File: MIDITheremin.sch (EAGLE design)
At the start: 104 parts, among them IC1 TL072P, IC2 TL072P, J1 DCJ0202, T1 2N3904, T2 2N3904, T3 2N3904, T4 2N3904, T5 2N3904

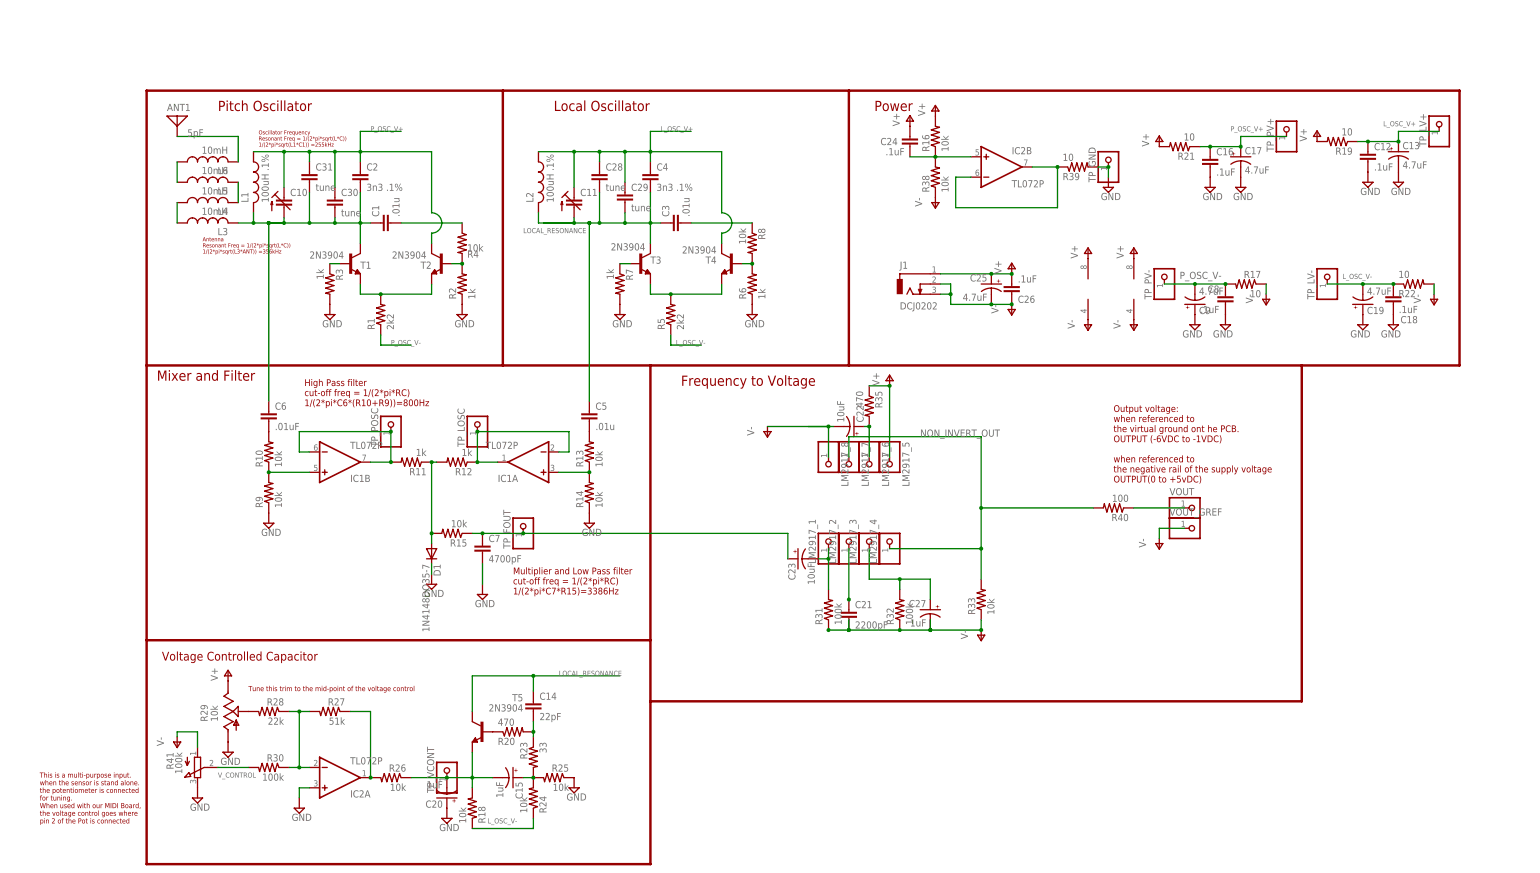
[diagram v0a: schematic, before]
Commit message: Add files via upload
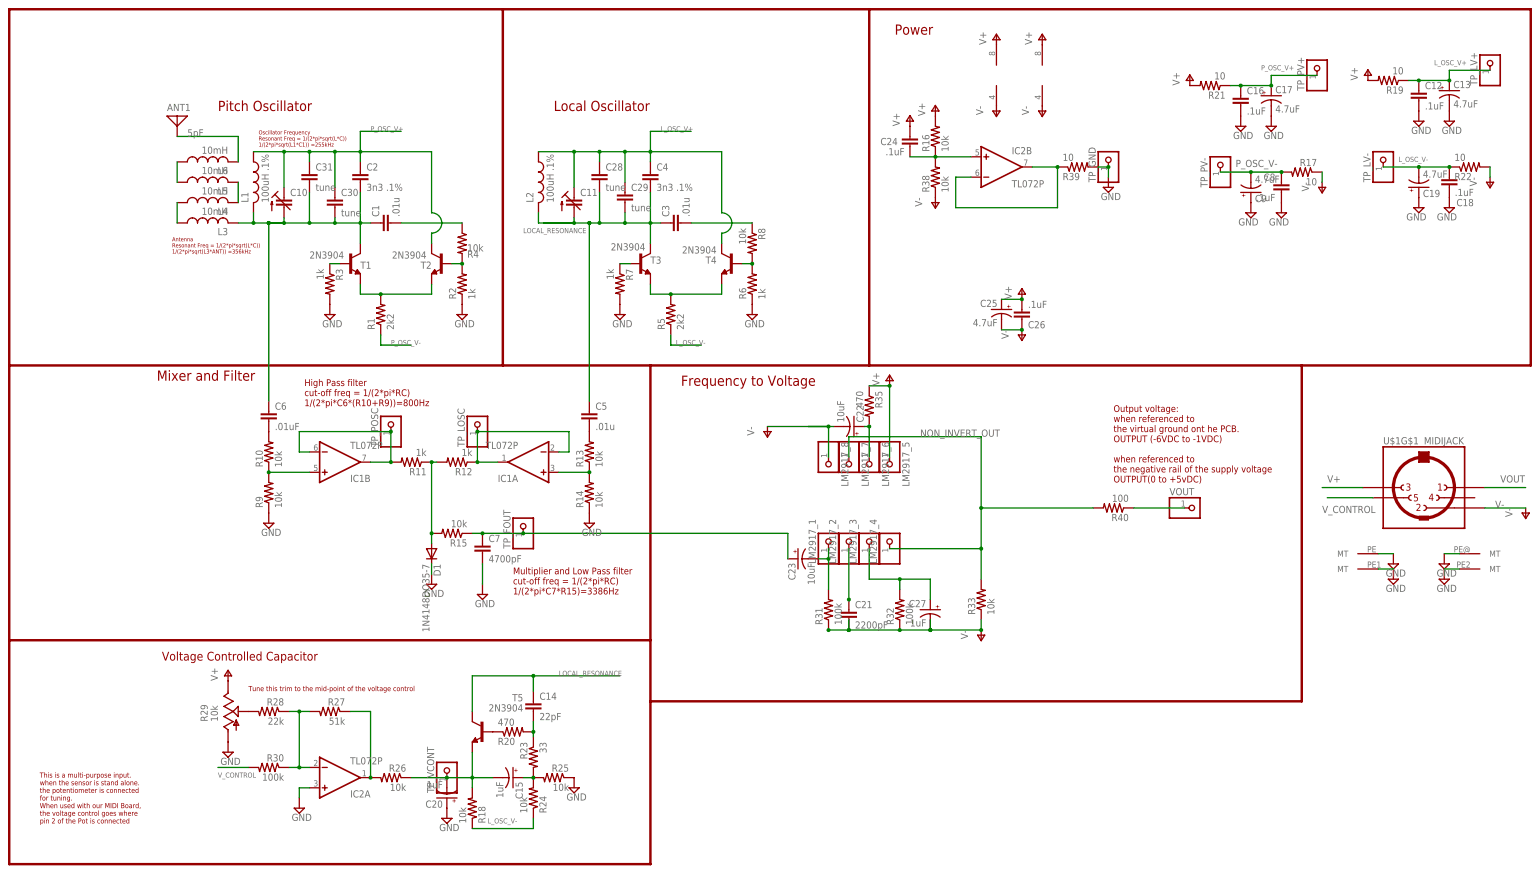
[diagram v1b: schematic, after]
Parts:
- removed J1: DCJ0202, con-jack:DCJ0202
- removed R41: 100k, pot:3RP/1610N
- removed VOUT_GREF: (no value), pinhead:PINHD-1X1
- added U$1: MIDIJACK, adafruit:MIDIJACK
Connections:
- removed net N$38: R40.1, VOUT.1
- new net VOUT: R40.1, U$1G$1.1, VOUT.1
- net GND: now also U$1G$2.MT, U$1G$3.MT, U$1G$4.MT, U$1G$5.MT; no longer R41.E
- net V+: now also U$1G$1.3; no longer J1.1
- net V-: now also U$1G$1.2; no longer J1.2, J1.3, R41.A, VOUT_GREF.1
- net V_CONTROL: now also U$1G$1.5; no longer R41.S
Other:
- moved on the sheet: C12, C13, C16, C17, C18, C19, C25, C26, C8, C9, R17, R19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
